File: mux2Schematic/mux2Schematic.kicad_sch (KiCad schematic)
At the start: 64 parts, among them J1 Conn_02x12_Odd_Even, J10 Conn_02x06_Top_Bottom, J11 Conn_02x06_Top_Bottom, J12 Conn_02x06_Top_Bottom, J13 Conn_02x06_Top_Bottom, J14 Conn_02x06_Top_Bottom, J15 Conn_01x02, J16 Conn_01x02, J17 Conn_01x02, J18 Conn_01x02, J19 Conn_01x02, J2 Conn_02x06_Top_Bottom, J20 Conn_01x02, J21 Conn_01x02, J3 Banana, J30 Conn_01x8, J31 Conn_01x8, J32 Conn_01x02, J33 Conn_01x02, J34 Conn_01x02, J35 Conn_01x02, J36 Conn_01x02, J37 Conn_01x02, J38 Conn_01x02, J39 Conn_01x02, J4 Banana, J5 Conn_01x8, J6 Conn_01x02, J7 Conn_02x06_Top_Bottom, J8 Conn_01x10, J9 Conn_02x06_Top_Bottom, U1 CD74HC4051E, U2 AMS1117-1.8, U3 AZ1084-3.3

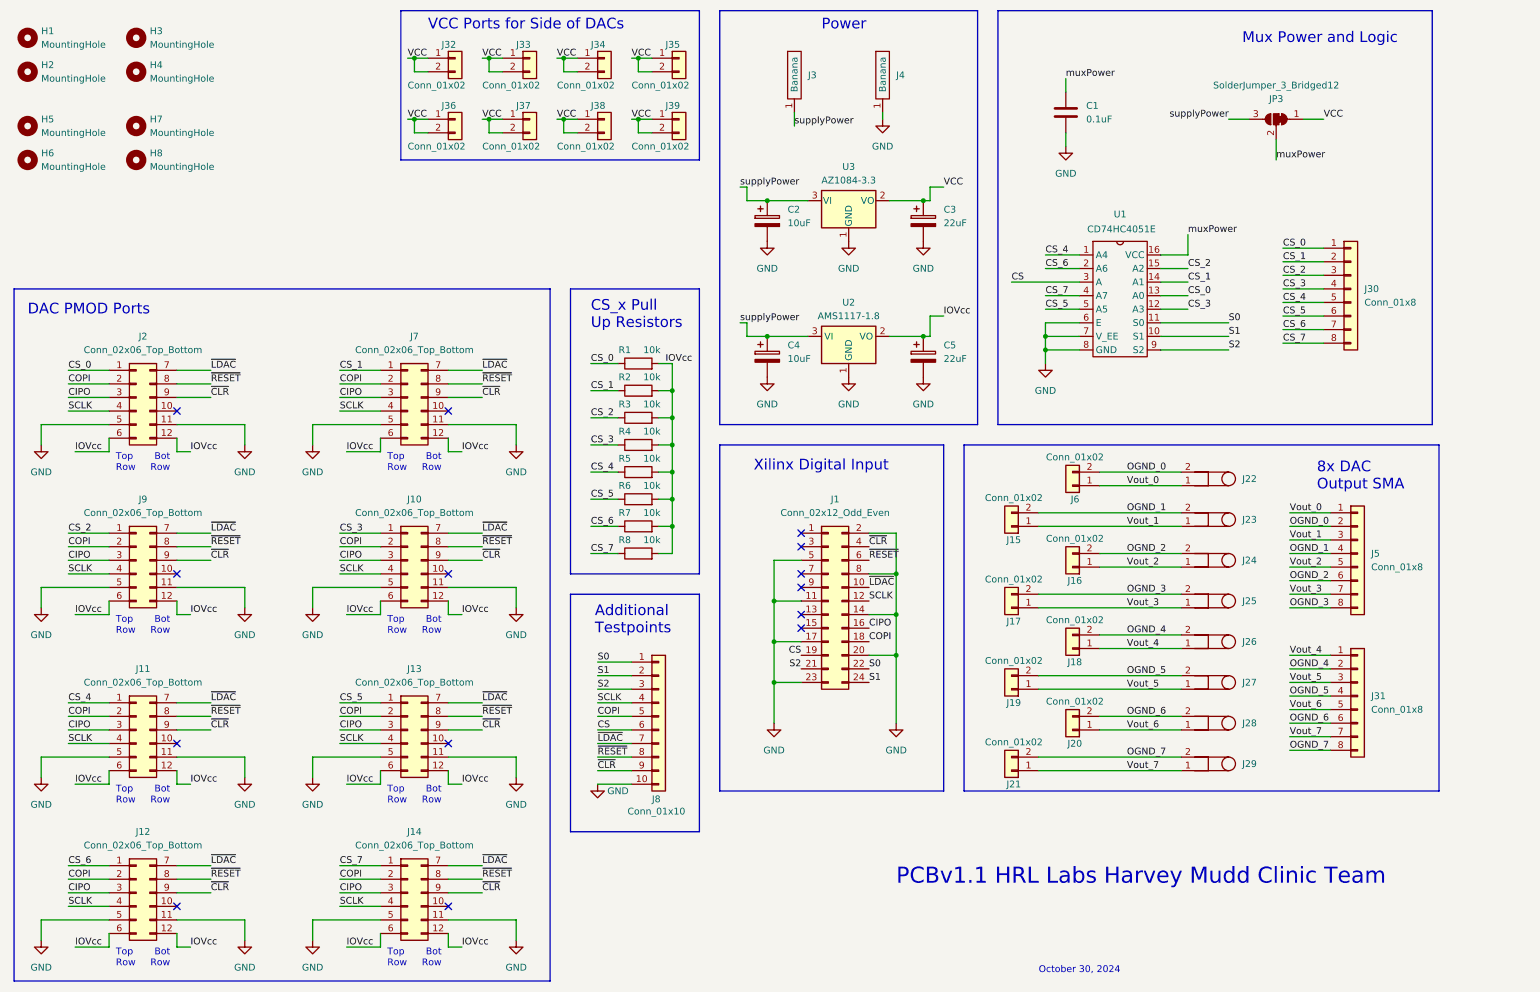
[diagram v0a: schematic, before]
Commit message: PCB finished!
Haven't thoroughly looked it over yet
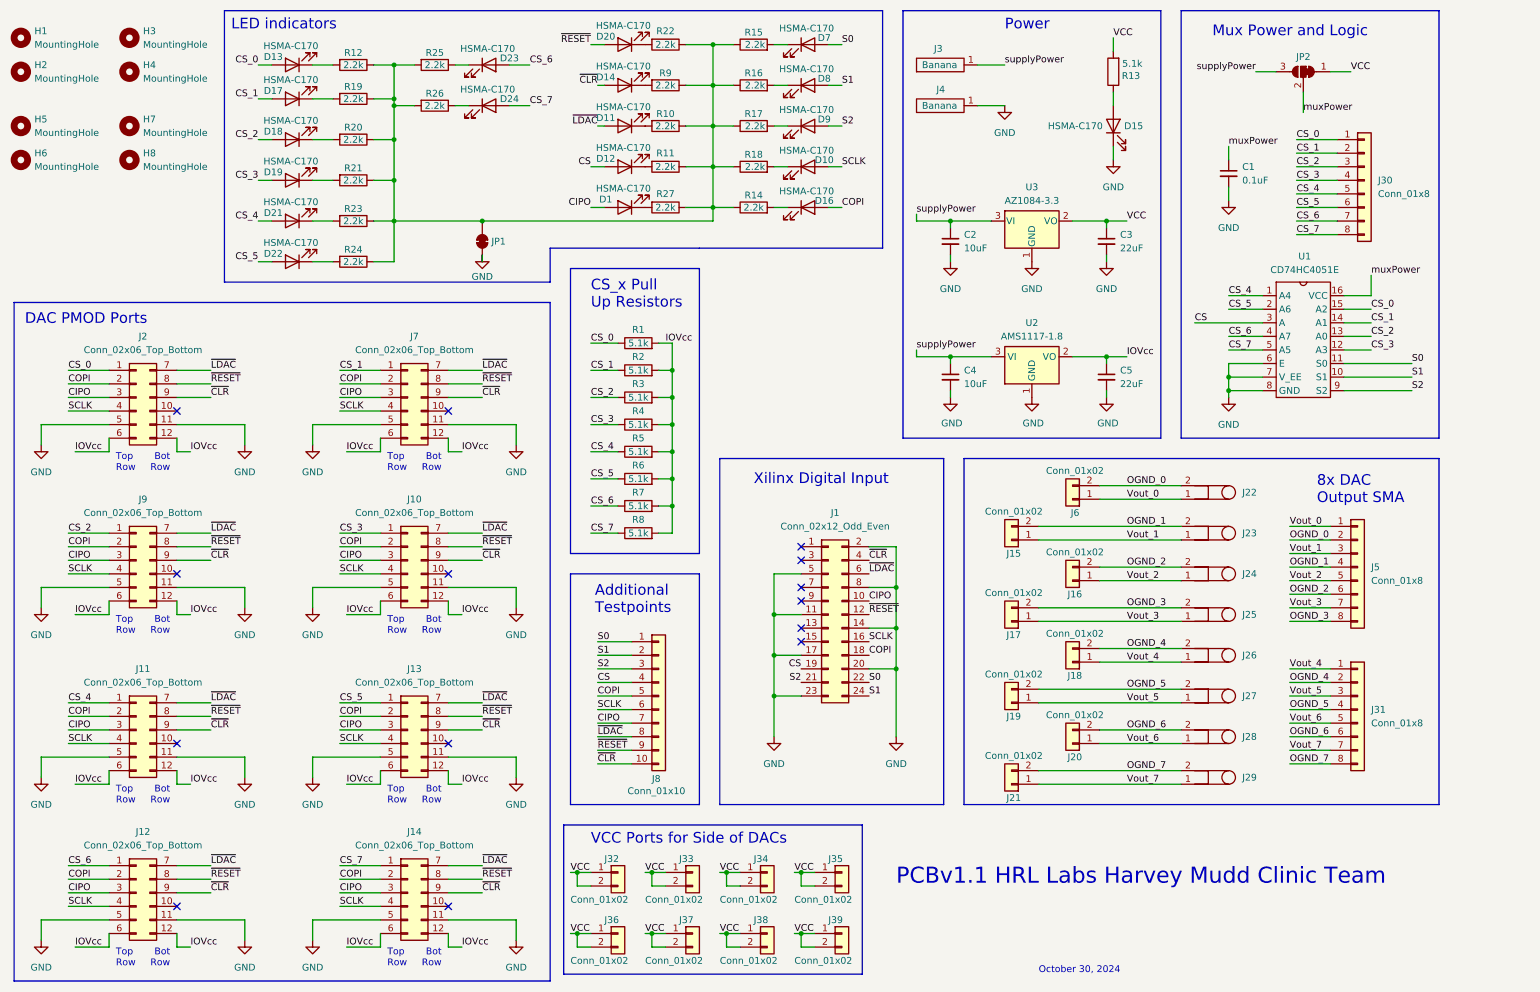
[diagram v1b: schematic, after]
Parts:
- added D1, D10, D11, D12, D13, D14, D15, D16, D17, D18, D19, D20, D21, D22, D23, D24, D7, D8, D9: HSMA-C170, LED_SMD:LED_0805_2012Metric, symbol Device:LED
- added JP1: SolderJumper_2_Bridged, Jumper:SolderJumper-2_P1.3mm_Bridged_RoundedPad1.0x1.5mm, symbol Jumper:SolderJumper_2_Bridged
- added R10, R11, R12, R14, R15, R16, R17, R18, R19, R20, R21, R22, R23, R24, R25, R26, R27, R9: 2.2k, Resistor_SMD:R_0805_2012Metric, symbol Device:R
- added R13: 5.1k, Resistor_SMD:R_0805_2012Metric, symbol Device:R
- C1: symbol Device:C -> Device:C_Small
- C2, C3, C4, C5: symbol Device:C_Polarized -> Device:C_Small
- R1, R2, R3, R4, R5, R6, R7, R8: value 10k -> 5.1k
- renumbered JP3 to JP2
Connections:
- net CIPO: now also J1.10 (Pin_10), J8.7 (Pin_7), D1.2 (A); no longer J1.16 (Pin_16)
- net COPI: now also D16.2 (A)
- net CS: now also J8.4 (Pin_4), D12.2 (A); no longer J8.6 (Pin_6)
- net CS_0: now also U1.15 (A2), D13.2 (A); no longer U1.13 (A0)
- net CS_1: now also D17.2 (A)
- net CS_2: now also U1.13 (A0), D18.2 (A); no longer U1.15 (A2)
- net CS_3: now also D19.2 (A)
- net CS_4: now also D21.2 (A)
- net CS_5: now also U1.2 (A6), D22.2 (A); no longer U1.5 (A5)
- net CS_6: now also U1.4 (A7), D23.2 (A); no longer U1.2 (A6)
- net CS_7: now also U1.5 (A5), D24.2 (A); no longer U1.4 (A7)
- net GND: now also D15.1 (K), JP1.1 (A); no longer J8.10 (Pin_10)
- net S0: now also D7.2 (A)
- net S1: now also D8.2 (A)
- net S2: now also D9.2 (A)
- net SCLK: now also J1.16 (Pin_16), J8.6 (Pin_6), D10.2 (A); no longer J1.12 (Pin_12), J8.4 (Pin_4)
- net VCC: now also R13.2
- net ~{CLR}: now also J8.10 (Pin_10), D14.2 (A); no longer J8.9 (Pin_9)
- net ~{LDAC}: now also J1.6 (Pin_6), J8.8 (Pin_8), D11.2 (A); no longer J1.10 (Pin_10), J8.7 (Pin_7)
- net ~{RESET}: now also J1.12 (Pin_12), J8.9 (Pin_9), D20.2 (A); no longer J1.6 (Pin_6), J8.8 (Pin_8)
- new net: JP1.2 (B), R10.1, R11.1, R12.1, R14.1, R15.1, R16.1, R17.1, R18.1, R19.1, R20.1, R21.1, R22.1, R23.1, R24.1, R25.2, R26.2, R27.1, R9.1
- new net: D7.1 (K), R15.2
- new net: D15.2 (A), R13.1
- new net: D10.1 (K), R18.2
- new net: D20.1 (K), R22.2
- new net: D23.1 (K), R25.1
- new net: D18.1 (K), R20.2
- new net: D9.1 (K), R17.2
- new net: D22.1 (K), R24.2
- new net: D16.1 (K), R14.2
- new net: D12.1 (K), R11.2
- new net: D13.1 (K), R12.2
- new net: D1.1 (K), R27.2
- new net: D11.1 (K), R10.2
- new net: D14.1 (K), R9.2
- new net: D24.1 (K), R26.1
- new net: D17.1 (K), R19.2
- new net: D8.1 (K), R16.2
- new net: D21.1 (K), R23.2
- new net: D19.1 (K), R21.2
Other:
- note added: "LED indicators"
- moved on the sheet: C1, H1, H2, H3, H4, H5, H6, H7, H8, J1, J15, J16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
